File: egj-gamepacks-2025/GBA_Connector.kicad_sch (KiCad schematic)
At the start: 6 parts, among them J5 GameBoy_GamePak_AGB-002, U10 SP3012-06UTG, U6 SP3012-06UTG, U7 SP3012-06UTG, U8 SP3012-06UTG, U9 SP3012-06UTG

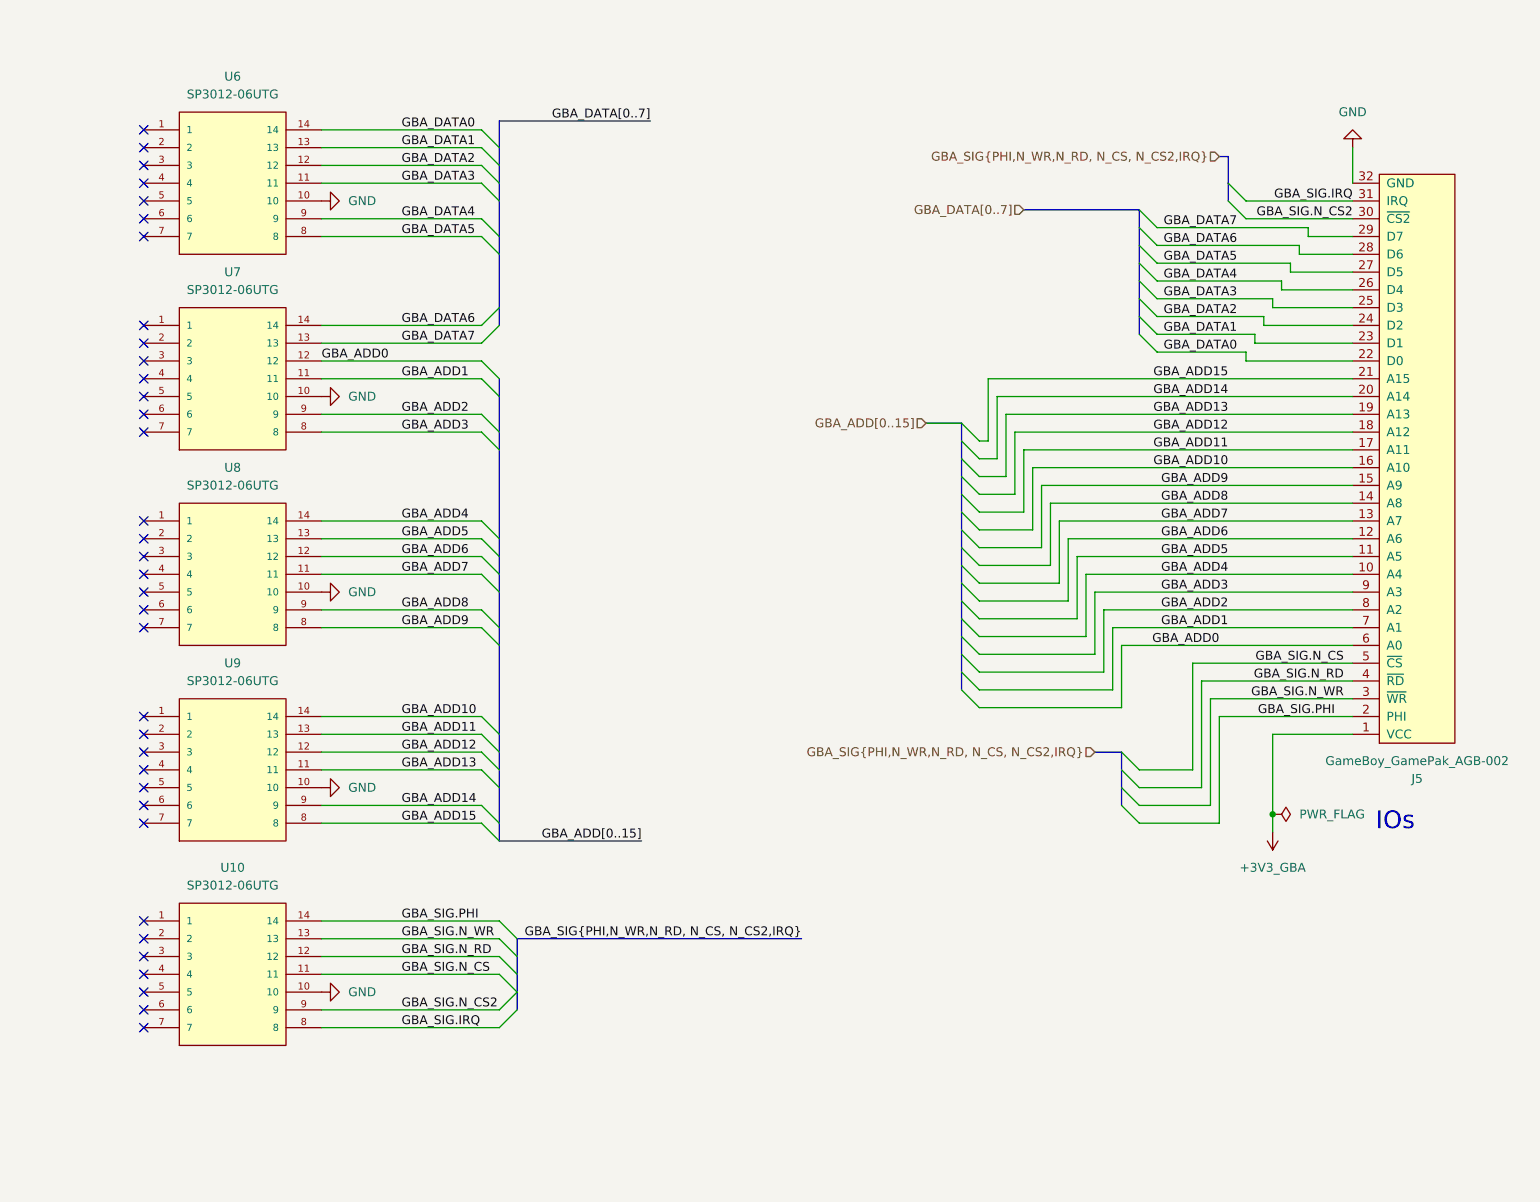
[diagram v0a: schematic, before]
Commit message: Update
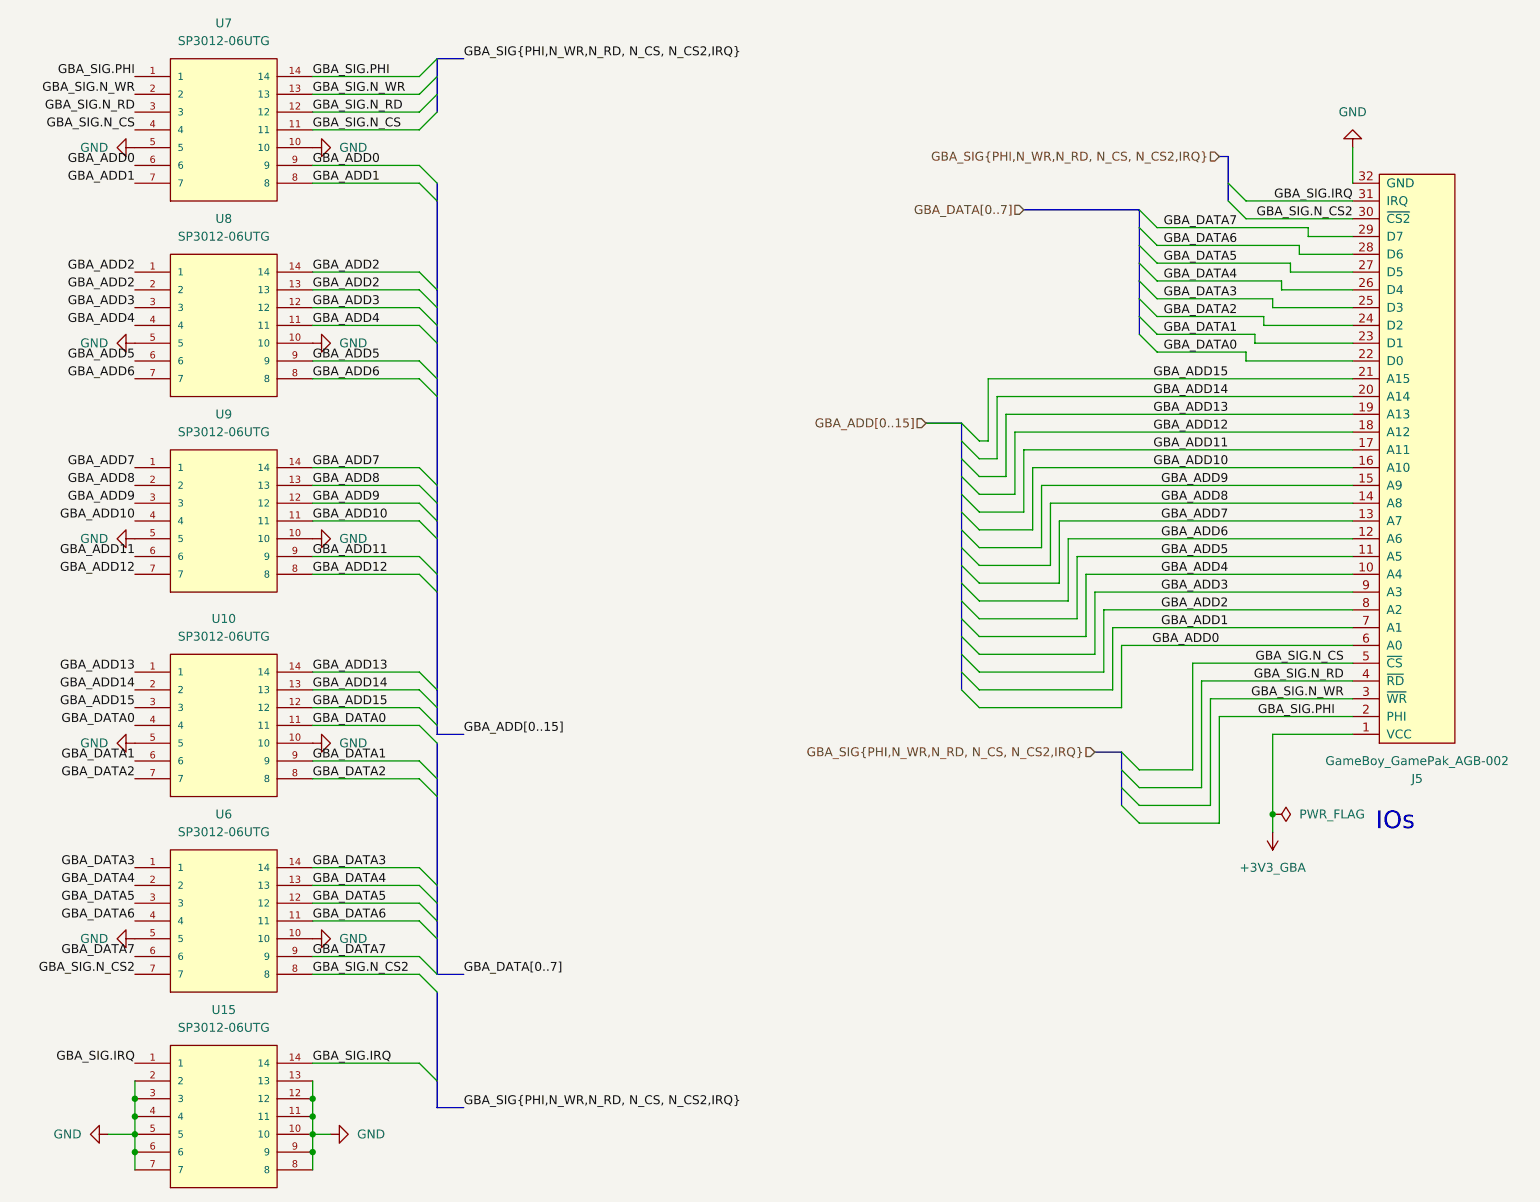
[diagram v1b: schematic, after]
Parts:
- added U15: SP3012-06UTG, Package_DFN_QFN:DFN-14_1.35x3.5mm_P0.5mm, symbol SP3012-06UTG:SP3012-06UTG
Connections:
- net GBA_ADD0: now also U7.6, U7.9; no longer U7.12
- net GBA_ADD1: now also U7.7, U7.8; no longer U7.11
- net GBA_ADD10: now also U9.11, U9.4; no longer U9.14
- net GBA_ADD11: now also U9.6, U9.9; no longer U9.13
- net GBA_ADD12: now also U9.7, U9.8; no longer U9.12
- net GBA_ADD13: now also U10.1, U10.14; no longer U9.11
- net GBA_ADD14: now also U10.13, U10.2; no longer U9.9
- net GBA_ADD15: now also U10.12, U10.3; no longer U9.8
- net GBA_ADD2: now also U8.1, U8.13, U8.14, U8.2; no longer U7.9
- net GBA_ADD3: now also U8.12, U8.3; no longer U7.8
- net GBA_ADD4: now also U8.11, U8.4; no longer U8.14
- net GBA_ADD5: now also U8.6, U8.9; no longer U8.13
- net GBA_ADD6: now also U8.7, U8.8; no longer U8.12
- net GBA_ADD7: now also U9.1, U9.14; no longer U8.11
- net GBA_ADD8: now also U9.13, U9.2; no longer U8.9
- net GBA_ADD9: now also U9.12, U9.3; no longer U8.8
- net GBA_DATA0: now also U10.11, U10.4; no longer U6.14
- net GBA_DATA1: now also U10.6, U10.9; no longer U6.13
- net GBA_DATA2: now also U10.7, U10.8; no longer U6.12
- net GBA_DATA3: now also U6.1, U6.14; no longer U6.11
- net GBA_DATA4: now also U6.13, U6.2; no longer U6.9
- net GBA_DATA5: now also U6.12, U6.3; no longer U6.8
- net GBA_DATA6: now also U6.11, U6.4; no longer U7.14
- net GBA_DATA7: now also U6.6, U6.9; no longer U7.13
- net GBA_SIG.IRQ: now also U15.1, U15.14; no longer U10.8
- net GBA_SIG.N_CS: now also U7.11, U7.4; no longer U10.11
- net GBA_SIG.N_CS2: now also U6.7, U6.8; no longer U10.9
- net GBA_SIG.N_RD: now also U7.12, U7.3; no longer U10.12
- net GBA_SIG.N_WR: now also U7.13, U7.2; no longer U10.13
- net GBA_SIG.PHI: now also U7.1, U7.14; no longer U10.14
- net GND: now also U10.5, U6.5, U7.5, U8.5, U9.5, U15.10, U15.11, U15.12, U15.13, U15.2, U15.3, U15.4, U15.5, U15.6, U15.7, U15.8, U15.9
- no-connect marks 35 -> 0
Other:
- moved on the sheet: U10, U6, U7, U8, U9
